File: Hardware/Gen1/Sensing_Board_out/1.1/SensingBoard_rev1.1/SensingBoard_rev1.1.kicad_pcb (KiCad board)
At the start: 6 copper layers, 40 x 40 mm, 89 parts, among them J1 USB_C_Receptacle, J2 3221-10-0300-00, J3 F32R-1A7H1-11024, J5 RS1-02-G, J6 RS1-02-G, J7 RS1-02-G, J9 RS1-02-G, SW1 PTS815 SJM 250 SMTR LFS, SW2 PTS815 SJM 250 SMTR LFS, U2 BNO055, U3 MIC5504-3.3YM5, U4 FT232RQ, U5 MIC5504-1.8YM5, U6 MCP1700x-280xxTT, U7 ESP32-S3, U8 GD25D05CT, Y1 ABM8G-40.000MHZ-18-D2Y-T

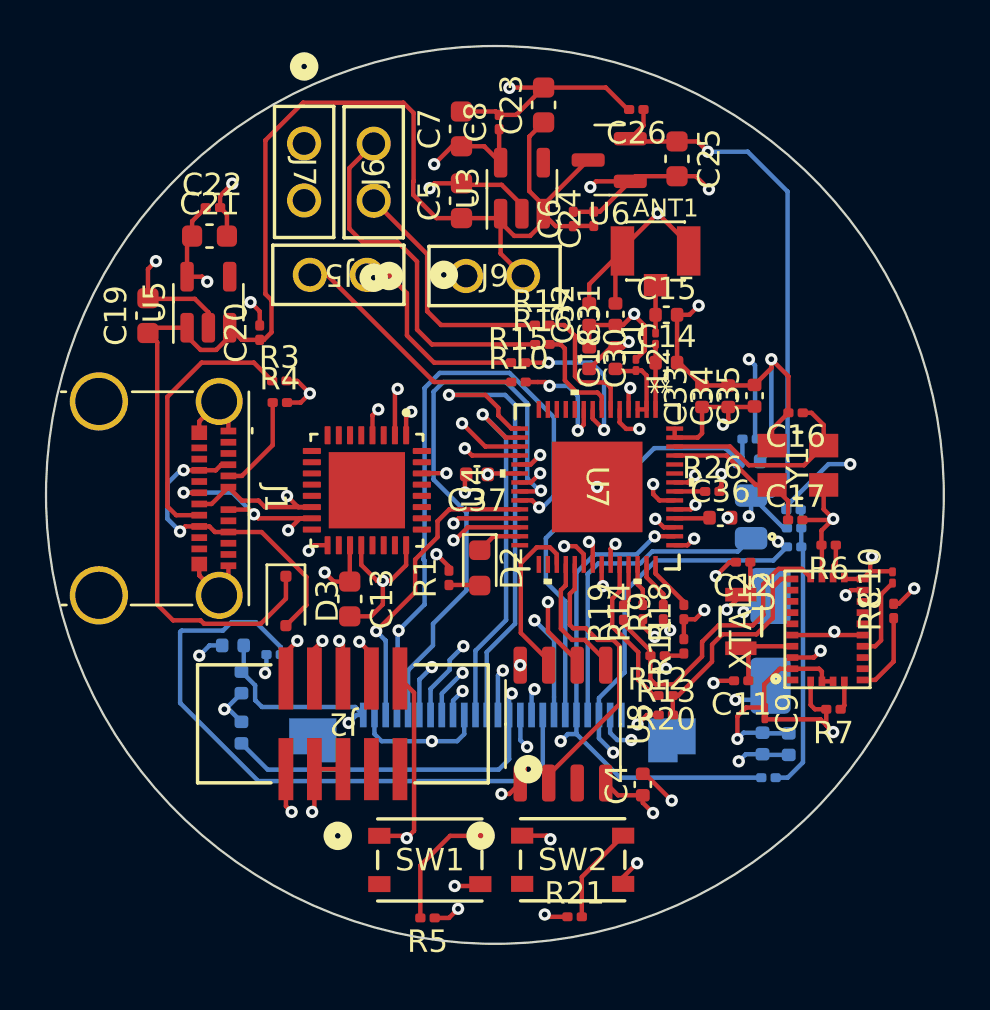
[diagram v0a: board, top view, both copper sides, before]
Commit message: fixed
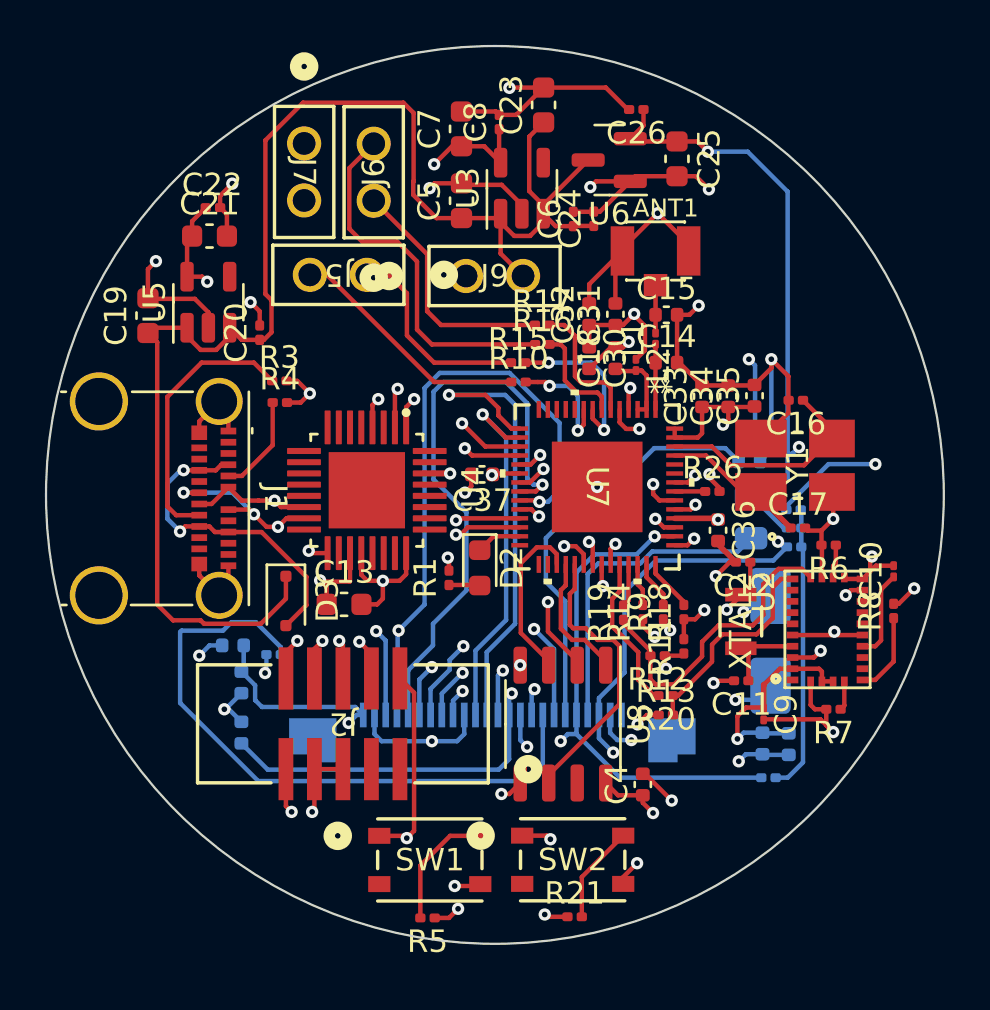
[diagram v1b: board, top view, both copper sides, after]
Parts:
- moved C36 0.57 mm to (140.1, 64.1), turned to -90 degrees
- moved C16 0.56 mm to (143.6, 58.3)
- moved C17 0.37 mm to (143.7, 64.0)
- moved C13 0.35 mm to (123.4, 67.4), turned to 0 degrees
- moved C10 0.28 mm to (147.9, 65.9)
- moved C37 0.23 mm to (129.6, 61.6)
- moved C9 0.07 mm to (142.1, 72.3)
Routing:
- net IO18/DVP_Y4: track 13.8 -> 34.4 mm, vias 1 -> 2
- net +2V8: track 61.4 -> 69.6 mm
- net +3.3V: track 51.8 -> 54.3 mm, vias 16 -> 17
- net USB_DP: track 18.7 -> 17.2 mm
- net USB_DN: track 19.9 -> 19.0 mm
- net GND: track 126.2 -> 125.7 mm, vias 36 -> 35
